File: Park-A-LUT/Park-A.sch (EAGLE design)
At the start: 41 parts, among them Q1 16MHz, T1 BC848SMD, T2 IRLML5203, T3 BC848SMD, T4 IRLML5203, U1 PIC18F25K80, U2 78M05, U3 TJA1055T

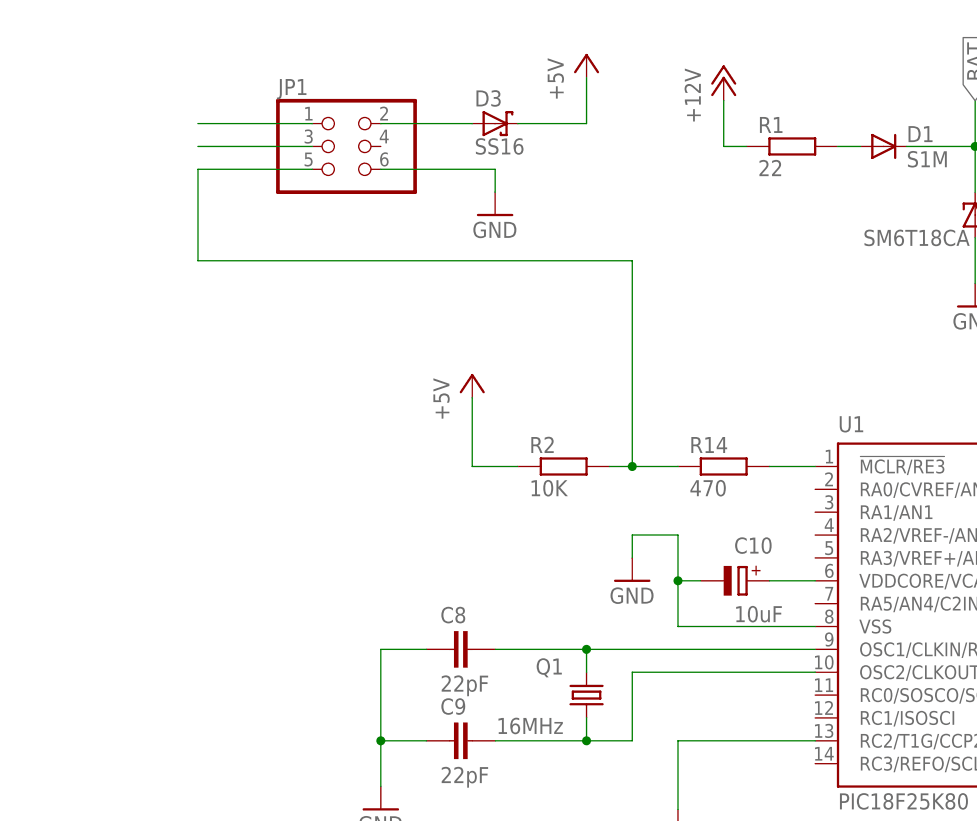
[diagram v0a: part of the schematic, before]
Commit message: Small fixes
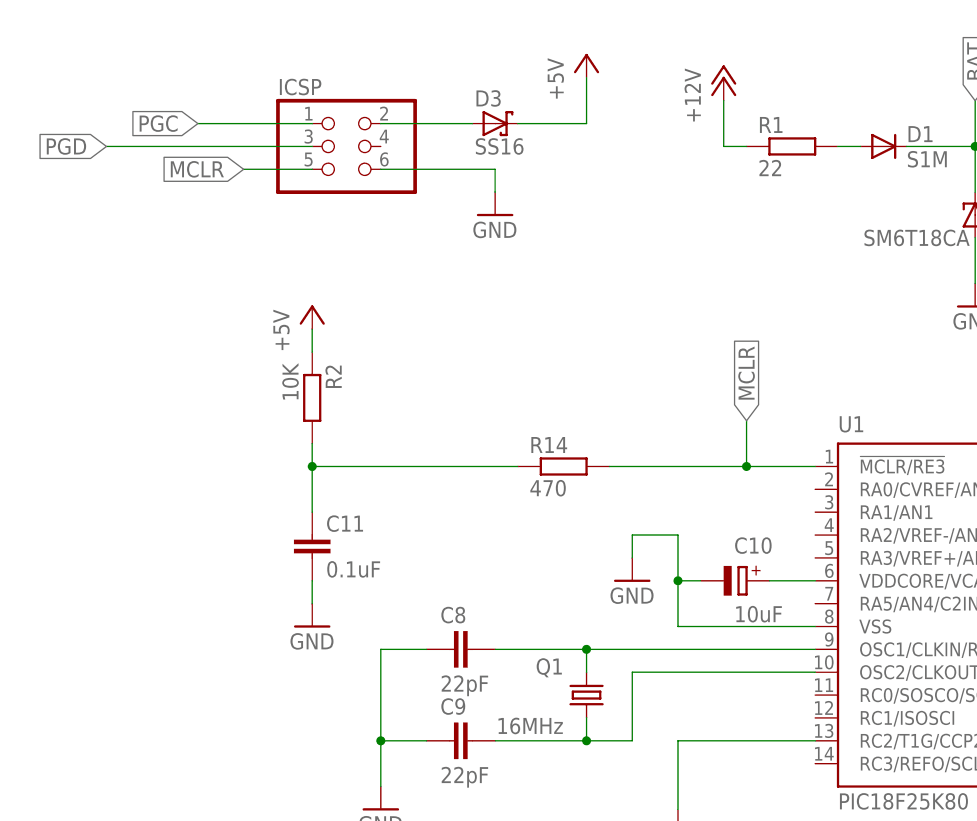
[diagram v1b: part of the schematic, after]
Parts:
- added C11: 0.1uF, rcl:C-EUC0805
- renumbered JP1 to ICSP
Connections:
- removed net N$19: ICSP.5, R14.1, R2.2
- new net MCLR: ICSP.5, R14.2, U1.!MCLR/RE3
- net GND: now also C11.2
- net N$4: now also C11.1, R14.1, R2.2; no longer R14.2, U1.!MCLR/RE3
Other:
- moved on the sheet: R14, R2
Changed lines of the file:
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@@
 <part name="T4" library="Park-A" deviceset="IRLML5203" device=""/>
 <part name="GND12" library="supply1" deviceset="GND" device=""/>
-<part name="JP1" library="Park-A" deviceset="PINHD-2X3" device=""/>
+<part name="ICSP" library="Park-A" deviceset="PINHD-2X3" device=""/>
 <part name="GND13" library="supply1" deviceset="GND" device=""/>
-<part name="R14" library="rcl" deviceset="R-EU_" device="R0805" value="470"/>
 <part name="D3" library="Park-A" deviceset="SS16" device=""/>
 <part name="P+6" library="supply1" deviceset="+5V" device=""/>
+<part name="R14" library="rcl" deviceset="R-EU_" device="R0805" value="470"/>
+<part name="C11" library="rcl" deviceset="C-EU" device="C0805" value="0.1uF"/>
+<part name="GND14" library="supply1" deviceset="GND" device=""/>
 </parts>
 <sheets>
@@
 <attribute name="NAME" x="86.36" y="-12.7" size="1.778" layer="94"/>
 </instance>
-<instance part="R2" gate="G$1" x="-96.52" y="-12.7"/>
-<instance part="P+3" gate="1" x="-106.68" y="-2.54"/>
+<instance part="R2" gate="G$1" x="-124.46" y="-5.08" rot="R270"/>
+<instance part="P+3" gate="1" x="-124.46" y="5.08"/>
 <instance part="P+4" gate="1" x="73.66" y="-2.54"/>
 <instance part="GND3" gate="1" x="58.42" y="-45.72"/>
@@
 <instance part="T4" gate="G$1" x="86.36" y="-73.66"/>
 <instance part="GND12" gate="1" x="5.08" y="-93.98"/>
-<instance part="JP1" gate="A" x="-121.92" y="22.86"/>
+<instance part="ICSP" gate="A" x="-121.92" y="22.86"/>
 <instance part="GND13" gate="1" x="-104.14" y="15.24"/>
-<instance part="R14" gate="G$1" x="-78.74" y="-12.7"/>
 <instance part="D3" gate="G$1" x="-104.14" y="25.4"/>
 <instance part="P+6" gate="1" x="-93.98" y="33.02"/>
+<instance part="R14" gate="G$1" x="-96.52" y="-12.7"/>
+<instance part="C11" gate="G$1" x="-124.46" y="-20.32"/>
+<instance part="GND14" gate="1" x="-124.46" y="-30.48"/>
 </instances>
 <busses>
@@
 </segment>
 <segment>
-<pinref part="JP1" gate="A" pin="6"/>
+<pinref part="ICSP" gate="A" pin="6"/>
 <pinref part="GND13" gate="1" pin="GND"/>
 <wire x1="-116.84" y1="20.32" x2="-104.14" y2="20.32" width="0.1524" layer="91"/>
 <wire x1="-104.14" y1="20.32" x2="-104.14" y2="17.78" width="0.1524" layer="91"/>
+</segment>
+<segment>
+<pinref part="GND14" gate="1" pin="GND"/>
+<pinref part="C11" gate="G$1" pin="2"/>
+<wire x1="-124.46" y1="-27.94" x2="-124.46" y2="-25.4" width="0.1524" layer="91"/>
 </segment>
 </net>
@@
 <segment>
 <pinref part="P+3" gate="1" pin="+5V"/>
-<wire x1="-106.68" y1="-5.08" x2="-106.68" y2="-12.7" width="0.1524" layer="91"/>
+<wire x1="-124.46" y1="2.54" x2="-124.46" y2="0" width="0.1524" layer="91"/>
 <pinref part="R2" gate="G$1" pin="1"/>
-<wire x1="-106.68" y1="-12.7" x2="-101.6" y2="-12.7" width="0.1524" layer="91"/>
 </segment>
 <segment>
@@
 </segment>
 <segment>
-<pinref part="JP1" gate="A" pin="1"/>
+<pinref part="ICSP" gate="A" pin="1"/>
 <wire x1="-124.46" y1="25.4" x2="-137.16" y2="25.4" width="0.1524" layer="91"/>
+<label x="-137.16" y="25.4" size="1.778" layer="95" rot="R180" xref="yes"/>
 </segment>
 </net>
@@
 </segment>
 <segment>
-<pinref part="JP1" gate="A" pin="3"/>
-<wire x1="-124.46" y1="22.86" x2="-137.16" y2="22.86" width="0.1524" layer="91"/>
-</segment>
-</net>
-<net name="N$19" class="0">
-<segment>
-<pinref part="JP1" gate="A" pin="5"/>
-<wire x1="-124.46" y1="20.32" x2="-137.16" y2="20.32" width="0.1524" layer="91"/>
-<wire x1="-137.16" y1="20.32" x2="-137.16" y2="10.16" width="0.1524" layer="91"/>
-<pinref part="R2" gate="G$1" pin="2"/>
-<wire x1="-88.9" y1="-12.7" x2="-91.44" y2="-12.7" width="0.1524" layer="91"/>
-<wire x1="-137.16" y1="10.16" x2="-88.9" y2="10.16" width="0.1524" layer="91"/>
-<wire x1="-88.9" y1="10.16" x2="-88.9" y2="-12.7" width="0.1524" layer="91"/>
-<pinref part="R14" gate="G$1" pin="1"/>
-<wire x1="-88.9" y1="-12.7" x2="-83.82" y2="-12.7" width="0.1524" layer="91"/>
-<junction x="-88.9" y="-12.7"/>
-</segment>
-</net>
-<net name="N$4" class="0">
-<segment>
+<pinref part="ICSP" gate="A" pin="3"/>
+<wire x1="-124.46" y1="22.86" x2="-147.32" y2="22.86" width="0.1524" layer="91"/>
+<label x="-147.32" y="22.86" size="1.778" layer="95" rot="R180" xref="yes"/>
+</segment>
+</net>
+<net name="MCLR" class="0">
+<segment>
+<wire x1="-76.2" y1="-7.62" x2="-76.2" y2="-12.7" width="0.1524" layer="91"/>
+<pinref part="U1" gate="G$1" pin="!MCLR/RE3"/>
+<wire x1="-76.2" y1="-12.7" x2="-68.58" y2="-12.7" width="0.1524" layer="91"/>
 <pinref part="R14" gate="G$1" pin="2"/>
-<pinref part="U1" gate="G$1" pin="!MCLR/RE3"/>
-<wire x1="-73.66" y1="-12.7" x2="-68.58" y2="-12.7" width="0.1524" layer="91"/>
+<wire x1="-91.44" y1="-12.7" x2="-76.2" y2="-12.7" width="0.1524" layer="91"/>
+<junction x="-76.2" y="-12.7"/>
+<label x="-76.2" y="-7.62" size="1.778" layer="95" rot="R90" xref="yes"/>
+</segment>
+<segment>
+<pinref part="ICSP" gate="A" pin="5"/>
+<wire x1="-124.46" y1="20.32" x2="-132.08" y2="20.32" width="0.1524" layer="91"/>
+<label x="-132.08" y="20.32" size="1.778" layer="95" rot="R180" xref="yes"/>
 </segment>
 </net>
 <net name="N$20" class="0">
 <segment>
-<pinref part="JP1" gate="A" pin="2"/>
+<pinref part="ICSP" gate="A" pin="2"/>
 <pinref part="D3" gate="G$1" pin="A"/>
 <wire x1="-116.84" y1="25.4" x2="-106.68" y2="25.4" width="0.1524" layer="91"/>
 </segment>
 </net>
+<net name="N$4" class="0">
+<segment>
+<pinref part="R2" gate="G$1" pin="2"/>
+<wire x1="-124.46" y1="-12.7" x2="-124.46" y2="-10.16" width="0.1524" layer="91"/>
+<pinref part="R14" gate="G$1" pin="1"/>
+<wire x1="-124.46" y1="-12.7" x2="-101.6" y2="-12.7" width="0.1524" layer="91"/>
+<pinref part="C11" gate="G$1" pin="1"/>
+<wire x1="-124.46" y1="-17.78" x2="-124.46" y2="-12.7" width="0.1524" layer="91"/>
+<junction x="-124.46" y="-12.7"/>
+</segment>
+</net>
